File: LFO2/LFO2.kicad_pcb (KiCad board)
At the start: 2 copper layers, 97.5 x 128 mm, 75 parts, among them J1 Conn_01x06_Female, J10 Conn_01x01_Pin, J11 Conn_01x01_Pin, J2 Conn_01x13_Pin, J3 Conn_01x13_Pin, J4 Conn_01x01_Pin, J5 Conn_01x01_Pin, J6 Conn_01x01_Pin, J7 Conn_01x01_Pin, J8 Conn_01x01_Pin, J9 Conn_01x01_Pin, Q1 BC557, Q2 BC547, Q3 BC557, Q4 BC547, SW1 SW_SPDT, SW2 SW_SPDT, U1 TL074, U12 Aux_flush, U13 Aux_flush, U15 Aux_flush, U16 Aux_flush, U2 DG417xJ, U3 Aux_flush, U4 TL072, U5 Aux_flush, U8 LM13700, U9 Aux_flush

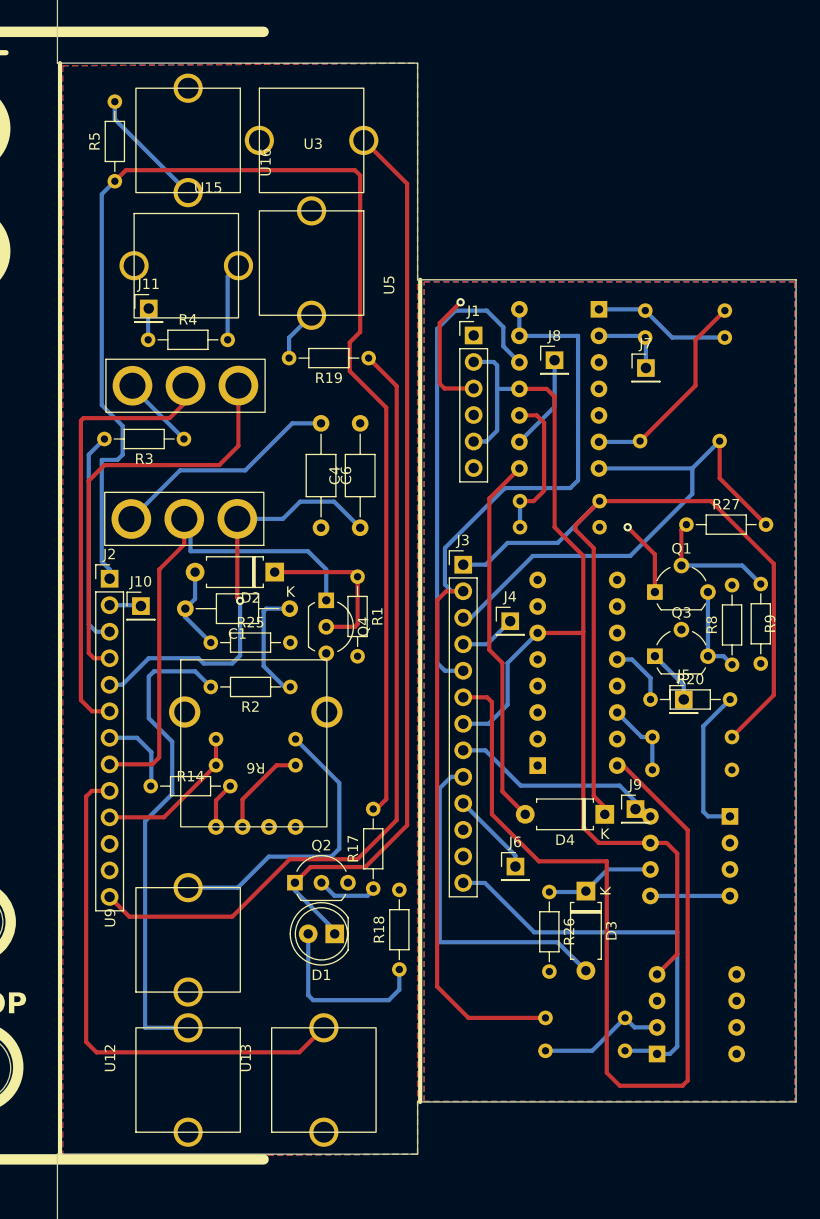
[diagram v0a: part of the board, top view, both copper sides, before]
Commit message: Add files via upload
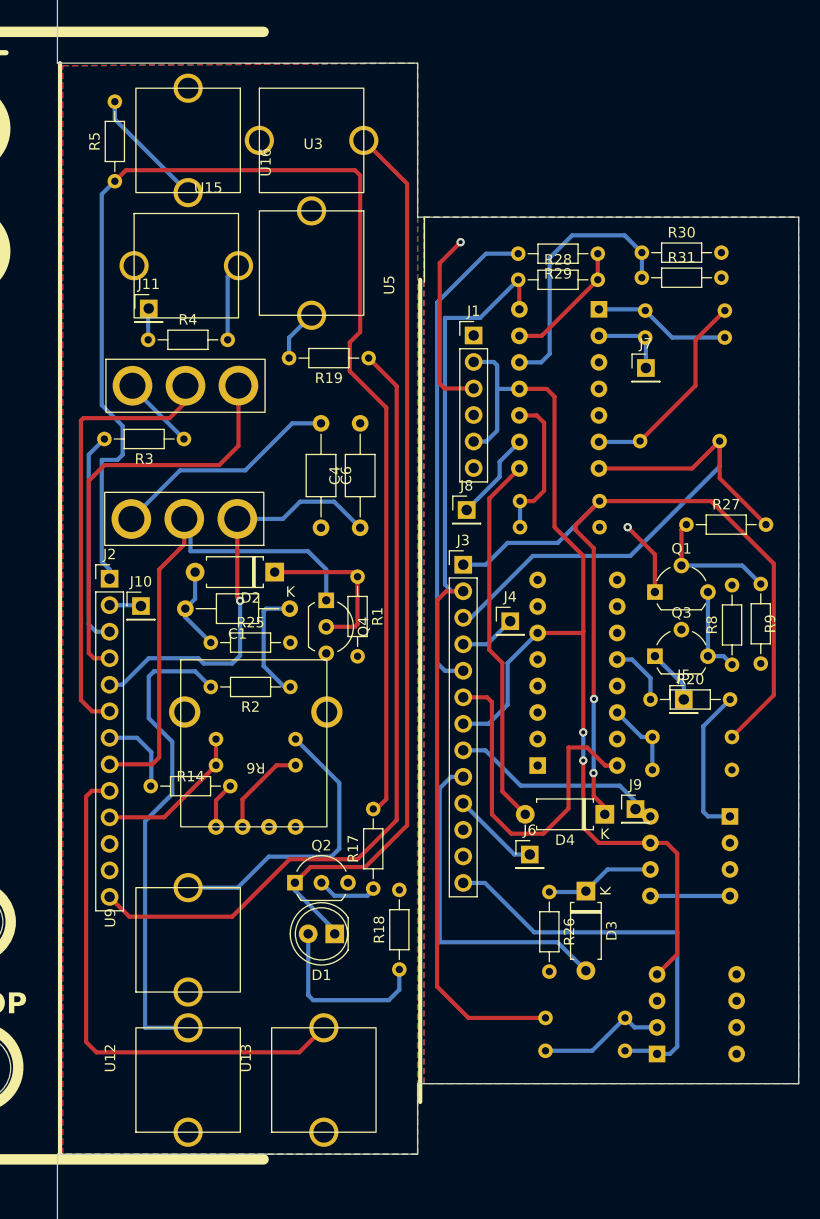
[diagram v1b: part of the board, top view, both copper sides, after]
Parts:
- added R28: 100k, Resistor_THT:R_Axial_DIN0204_L3.6mm_D1.6mm_P7.62mm_Horizontal, F.Cu at (117.9, 73.5)
- added R29: 100k, Resistor_THT:R_Axial_DIN0204_L3.6mm_D1.6mm_P7.62mm_Horizontal, F.Cu at (125.5, 71.0)
- added R30: 100k, Resistor_THT:R_Axial_DIN0204_L3.6mm_D1.6mm_P7.62mm_Horizontal, F.Cu at (129.7, 70.9)
- added R31: 100k, Resistor_THT:R_Axial_DIN0204_L3.6mm_D1.6mm_P7.62mm_Horizontal, F.Cu at (129.7, 73.3)
- moved J8 16.6 mm to (113.0, 95.5)
- moved J6 1.80 mm to (119.0, 128.6)
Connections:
- U1 pad 12: CAP -> Net-(U1D-+)
- U1 pad 13: TRI -> Net-(U1D--)
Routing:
- net ABC: track 130.9 -> 76.9 mm
- net Net-(U1D-+): track 0.00 -> 25.2 mm
- net Net-(U1D--): track 0.00 -> 12.2 mm
- net GND: track 19.4 -> 25.1 mm
- net TRI: track 100.5 -> 96.5 mm
- net CV1: track 72.4 -> 76.1 mm
- net SW: track 78.7 -> 78.1 mm
- net SQR: vias 0 -> 2
- net -12V: vias 0 -> 2
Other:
- board size 97.5 x 128 mm -> 97.8 x 128 mm

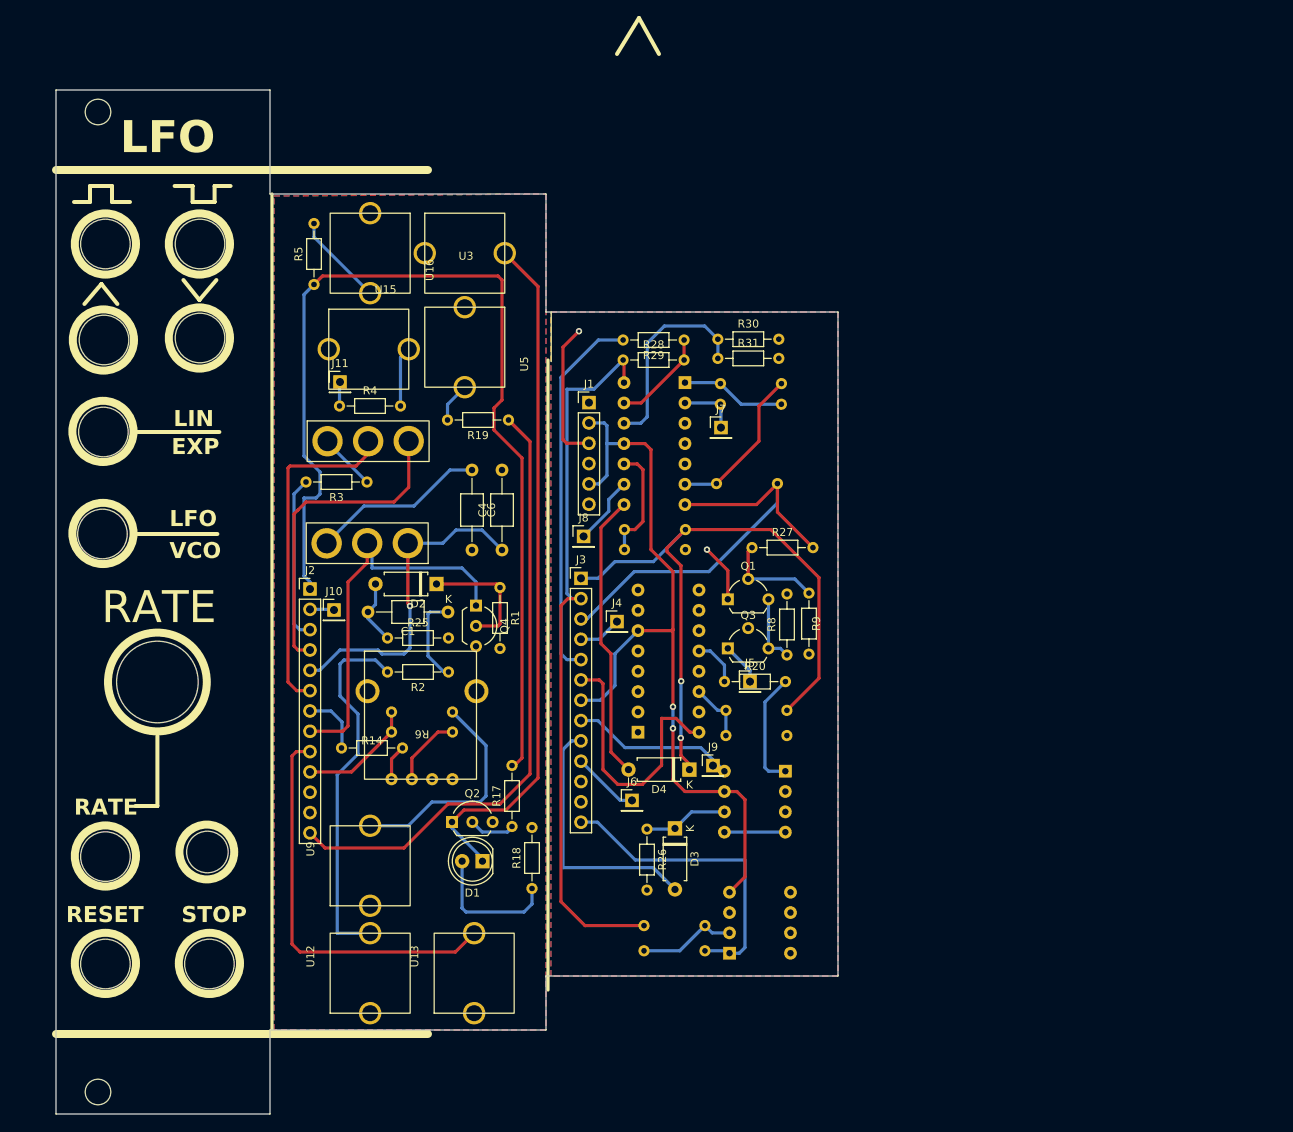
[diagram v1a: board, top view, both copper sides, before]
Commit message: Add files via upload
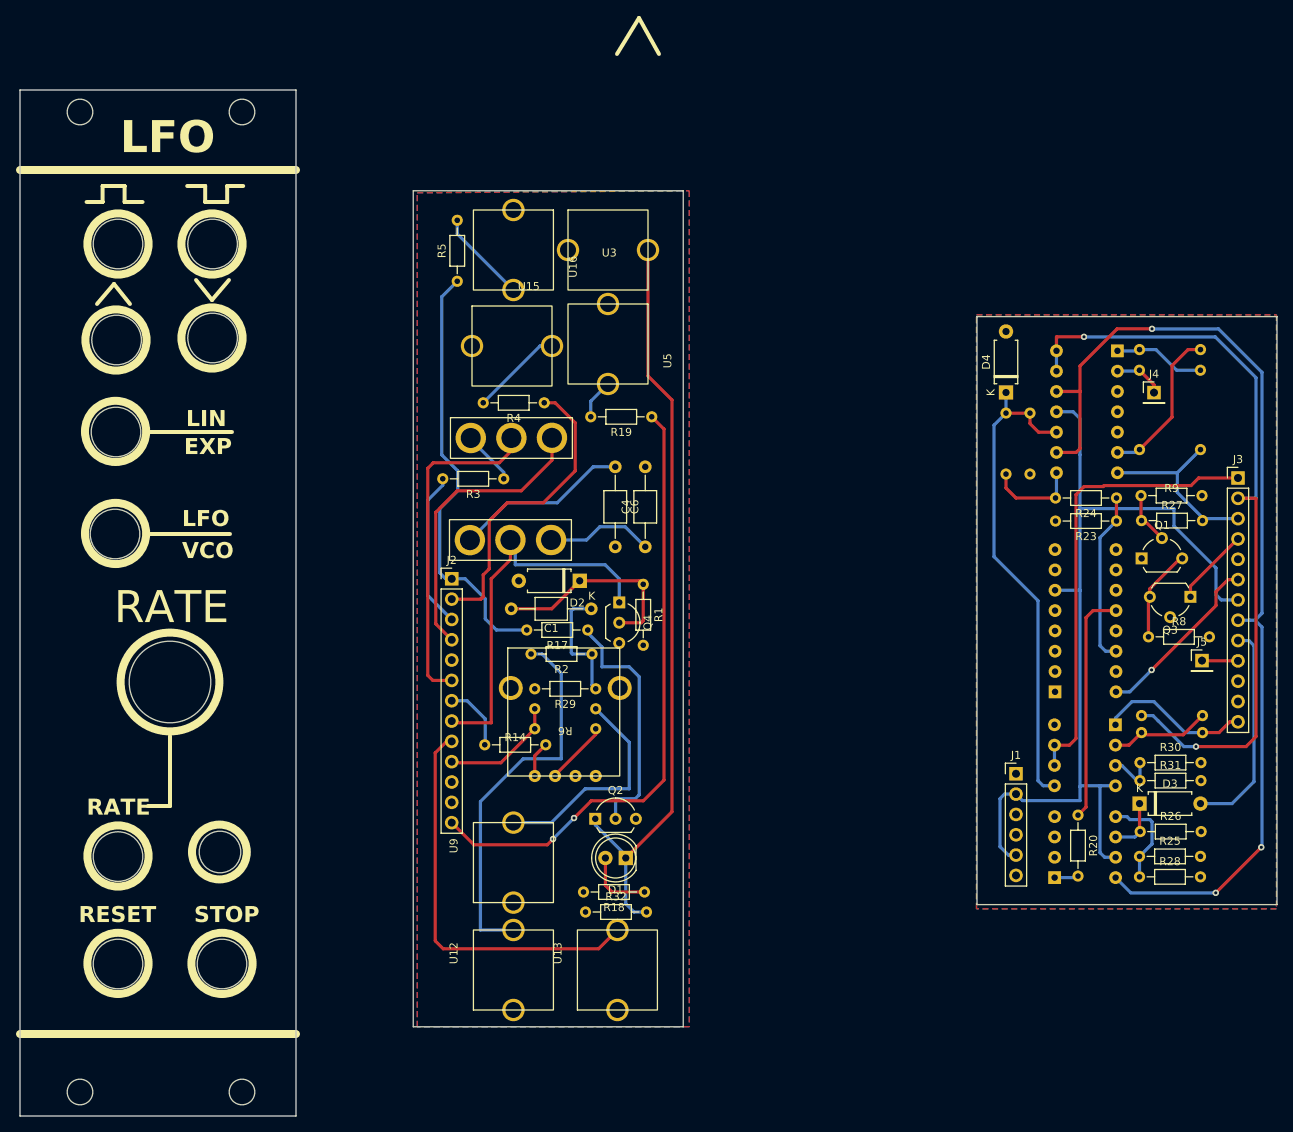
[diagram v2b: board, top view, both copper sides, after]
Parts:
- removed J10, J11, J6, J7, J8, J9: Conn_01x01_Pin, Connector_PinHeader_2.54mm:PinHeader_1x01_P2.54mm_Vertical
- added R32: 4k7, Resistor_THT:R_Axial_DIN0204_L3.6mm_D1.6mm_P7.62mm_Horizontal, F.Cu at (113.2, 142.5)
- added REF**: MountingHole_3.2mm_M3, MountingHole:MountingHole_3.2mm_M3, F.Cu at (70.2, 165.0)
- added REF**: MountingHole_3.2mm_M3, MountingHole:MountingHole_3.2mm_M3, F.Cu at (70.2, 42.5)
- R23, R24: moved to F.Cu
- moved R25 97.9 mm to (182.4, 135.6)
- moved R28 91.3 mm to (182.4, 138.1)
- moved J3 83.1 mm to (194.8, 88.2)
- moved R30 74.7 mm to (182.5, 123.8)
- moved R31 74.6 mm to (182.5, 126.1)
- moved J4 73.0 mm to (184.2, 77.6)
- moved J1 70.7 mm to (167.0, 125.2)
- moved R16 67.9 mm to (190.3, 120.1)
- moved R7 67.5 mm to (190.3, 118.0)
- moved R26 61.7 mm to (182.5, 132.4), turned to 0 degrees
- moved D4 61.5 mm to (165.8, 77.6), turned to 90 degrees
- moved Q3 58.2 mm to (188.8, 103.1), turned to 180 degrees
- moved D3 58.2 mm to (182.4, 128.9), turned to 0 degrees
- moved J5 56.6 mm to (190.2, 111.1)
- moved U4 56.1 mm to (179.4, 119.1), turned to 180 degrees
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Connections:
- C1 pad 2: Net-(D2-A) -> Net-(D2-K)
- C4 pad 1: CAP -> Net-(SW1-A)
- D2 pad 2: Net-(D2-A) -> GND
- D4 pad 1: SQR -> Net-(D4-K)
- D4 pad 2: Net-(D4-A) -> GND
- J2 pad 5: CAP -> unconnected-(J2-Pin_5-Pad5)
- J3 pad 5: CAP -> unconnected-(J3-Pin_5-Pad5)
- J4 pad 1: CV2 -> VGND
- J5 pad 1: CV2 -> VGND
- R21 pad 1: SQR -> Net-(R21-Pad1)
- R21 pad 2: Net-(U1C-+) -> Net-(D4-K)
- R22 pad 1: Net-(U1C-+) -> Net-(D4-K)
- R24 pad 2: SQR -> Net-(R21-Pad1)
- R25 pad 1: Net-(D2-A) -> Net-(U2B-VL)
- R25 pad 2: GND -> +12V
- R28 pad 1: TRI -> Net-(U2B-VL)
- R28 pad 2: Net-(U1D--) -> GND
- R29 pad 1: Net-(U1D--) -> Net-(C1-Pad1)
- R29 pad 2: CAP -> GND
- R30 pad 1: Net-(U1D-+) -> Net-(U4A-+)
- R31 pad 1: Net-(U1D-+) -> Net-(U4A-+)
- SW1 pad 1: CAP -> Net-(SW1-A)
- U1 pad 10: Net-(U1C-+) -> Net-(D4-K)
- U1 pad 12: Net-(U1D-+) -> SW
- U1 pad 13: Net-(U1D--) -> TRI
- U1 pad 8: Net-(D4-A) -> Net-(R21-Pad1)
- U2 pad 5: +12V -> Net-(U2B-VL)
- U4 pad 3: GND -> Net-(U4A-+)
- U4 pad 5: unconnected-(U4B-+-Pad5) -> Net-(D4-K)
- U4 pad 6: unconnected-(U4B---Pad6) -> SQR
- U4 pad 7: unconnected-(U4-Pad7) -> SQR
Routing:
- net SQR: track 214.0 -> 111.5 mm, vias 2 -> 0
- net SW: track 78.1 -> 175.8 mm, vias 0 -> 3
- net CAP: track 87.4 -> 0.00 mm, vias 1 -> 0
- net Net-(D4-K): track 0.00 -> 61.8 mm
- net TRI: track 96.5 -> 135.2 mm, vias 0 -> 2
- net Net-(D4-A): track 35.7 -> 0.00 mm
- net CV1: track 76.1 -> 43.0 mm
- net Net-(U1D-+): track 25.2 -> 0.00 mm
- net GND: track 25.1 -> 0.00 mm, vias 2 -> 0
- net Net-(Q2-B): track 5.71 -> 30.8 mm
- net Net-(R20-Pad1): track 5.98 -> 29.2 mm
- net ITRI: track 116.3 -> 96.2 mm, vias 0 -> 2
- net -12V: track 107.3 -> 124.3 mm, vias 2 -> 0
- net Net-(U1C-+): track 14.4 -> 0.00 mm
- net Net-(U8A-+): track 7.49 -> 21.6 mm
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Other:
- board size 97.8 x 128 mm -> 157.1 x 128.2 mm
